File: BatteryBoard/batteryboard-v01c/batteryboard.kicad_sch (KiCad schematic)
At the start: 30 parts, among them J1 KEYSTONE-1042, J2 KEYSTONE-1042, J3 KEYSTONE-1042, J4 KEYSTONE-1042, J5 KEYSTONE-1042, J6 KEYSTONE-1042, J7 MOLEX 5023520601, J8 Screw_Terminal_01x02, Q1 IRF7458, Q2 IRF7458, Q3 MMBT2222AT, U1 R5460N233AF

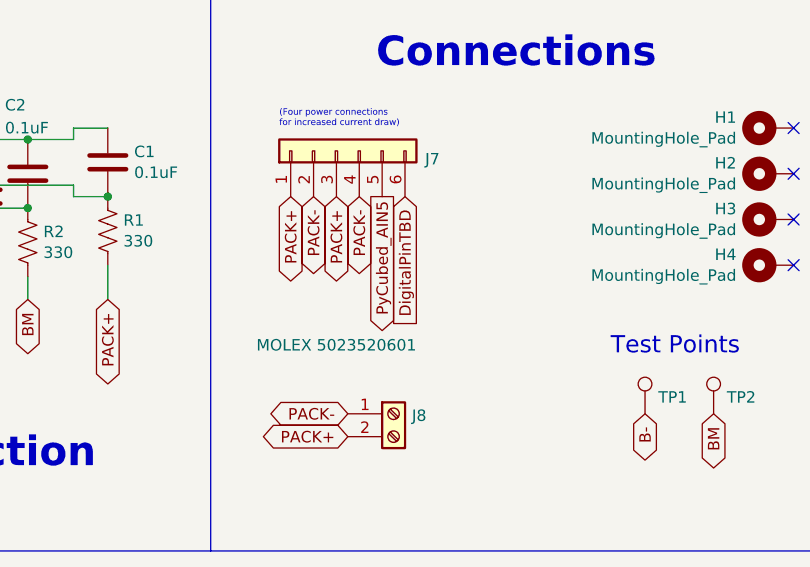
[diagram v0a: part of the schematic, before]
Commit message: final silkscreen and stencil edits, gerbers added for final purchase
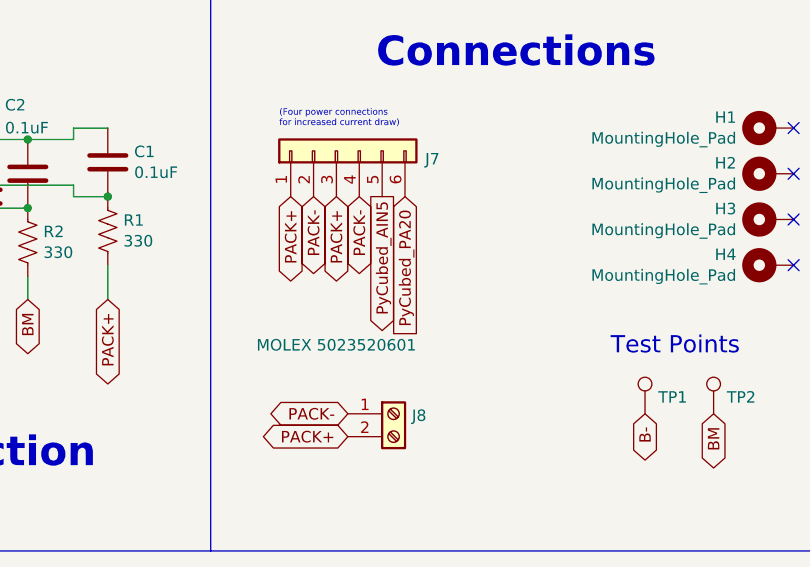
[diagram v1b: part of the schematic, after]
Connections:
- net DigitalPinTBD is gone; now on net PyCubed_PA20: J7.6 (Pin_6)
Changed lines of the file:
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@@
     )
   )
-  (global_label "DigitalPinTBD" (shape input) (at 218.44 95.25 270) (fields_autoplaced)
+  (global_label "PyCubed_PA20" (shape input) (at 218.44 95.25 270) (fields_autoplaced)
     (effects (font (size 1.27 1.27)) (justify right))
-    (property "Intersheet References" "${INTERSHEET_REFS}" (id 0) (at 0 0 0)
-      (effects (font (size 1.27 1.27)) hide)
+    (property "Intersheet References" "${INTERSHEET_REFS}" (id 0) (at 218.3606 111.3628 90)
+      (effects (font (size 1.27 1.27)) (justify right) hide)
     )
   )
